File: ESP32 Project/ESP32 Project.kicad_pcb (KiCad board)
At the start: 4 copper layers, 89.5 x 55 mm, 87 parts, among them J1 2338792-1, J2 B2B-PH-SM4-TB, J3 GSD090012SEU, J4 Conn_01x04_Pin, J5 Conn_01x05_Pin, Q1 TEMT6000X01, Q2 BC817, Q3 BC817, U1 MCP73871, U2 W25Q32JVSSIQ, U3 ESP32-C3-WROOM-02-H4, U4 CP2102N-Axx-xQFN20, U5 USBLC6-2SC6, U6 BME280, U7 MAX4466EXK

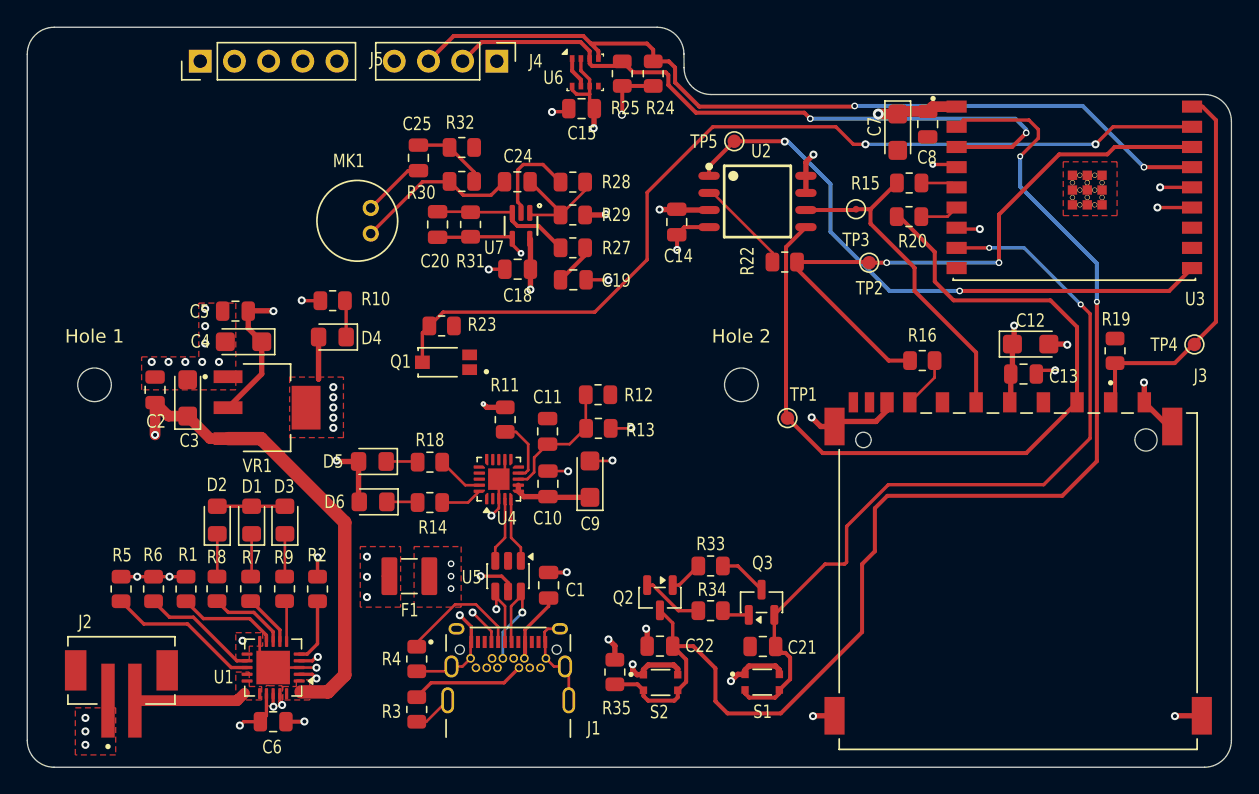
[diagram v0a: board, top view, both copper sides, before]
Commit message: pcb tomoroow is gonna be done
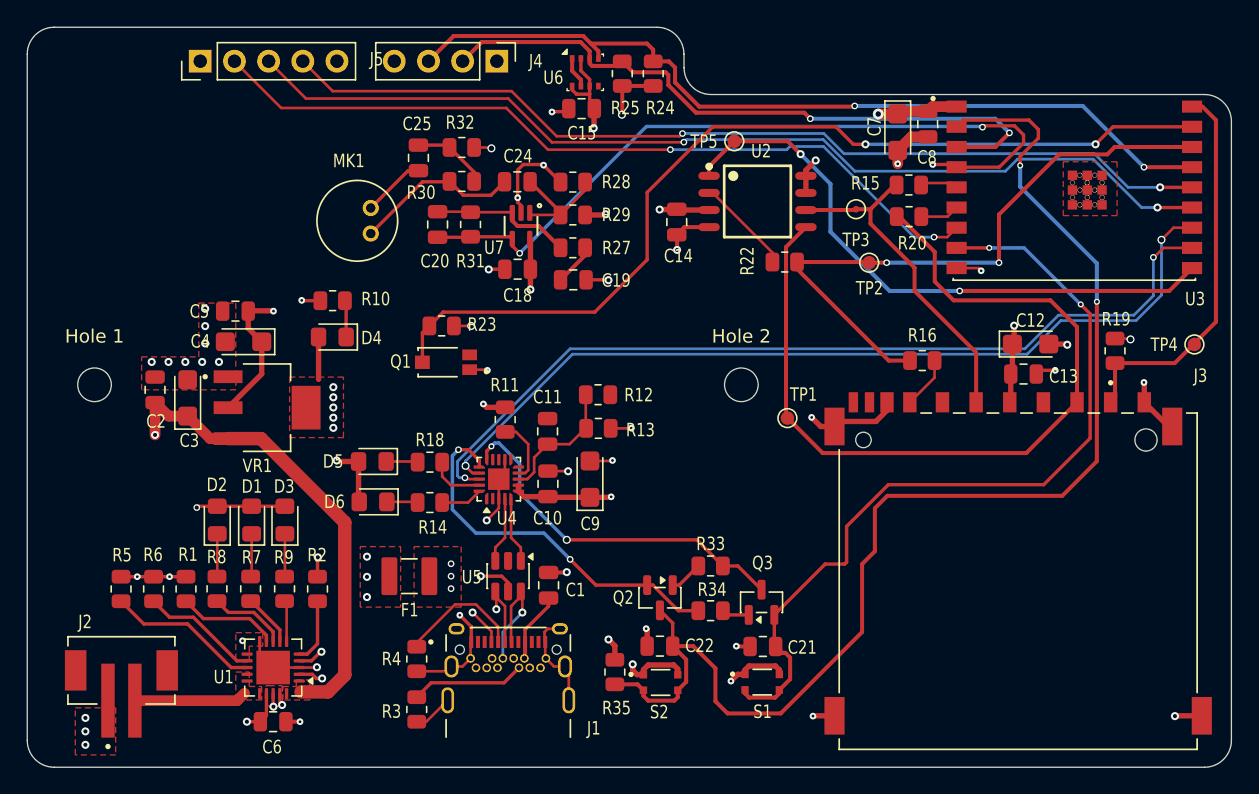
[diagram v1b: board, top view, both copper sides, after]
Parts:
- moved R20 0.15 mm to (242.5, 71.7)
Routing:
- net /Esp32-C2-02/TX-RX: track 0.00 -> 65.7 mm, vias 0 -> 2
- net /Esp32-C2-02/RX-TX: track 0.00 -> 65.2 mm, vias 0 -> 2
- net /Esp32-C2-02/MIC-OUT: track 8.83 -> 56.8 mm, vias 2 -> 3
- net /Esp32-C2-02/RTS: track 4.59 -> 28.4 mm, vias 0 -> 2
- net /Esp32-C2-02/DTR: track 3.61 -> 27.1 mm, vias 0 -> 2
- net GND: track 96.5 -> 104.7 mm, vias 37 -> 43
- net /Esp32-C2-02/GPIO8: track 64.9 -> 59.7 mm, vias 1 -> 2
- net +3.3V: track 63.7 -> 68.7 mm, vias 17 -> 21
- net /Esp32-C2-02/SDA: track 52.3 -> 49.6 mm
- net /Esp32-C2-02/GPIO19: track 72.1 -> 70.1 mm, vias 1 -> 2
- net /5volt usb: track 14.2 -> 16.0 mm, vias 8 -> 9
- net Net-(U4-~{RXT}/GPIO.3): track 3.47 -> 4.09 mm
- net /Esp32-C2-02/GPIO18: track 74.4 -> 74.1 mm, vias 1 -> 2
- added copper zone on In2.Cu, net +3.3V
- added copper zone on In2.Cu, net /5volt usb
- added copper zone on In1.Cu, net GND
- added copper zone on In2.Cu, net VBUS_A
- removed copper zone on In1.Cu, net +3.3V
- removed copper zone on In1.Cu, net /+5Volt
- removed copper zone on In1.Cu, net /5volt usb
- removed copper zone on In2.Cu, net GND
- removed copper zone on In1.Cu, net VBUS_A
